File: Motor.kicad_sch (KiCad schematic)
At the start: 38 parts, among them U1 MCF8315C1VQRGFRQ1

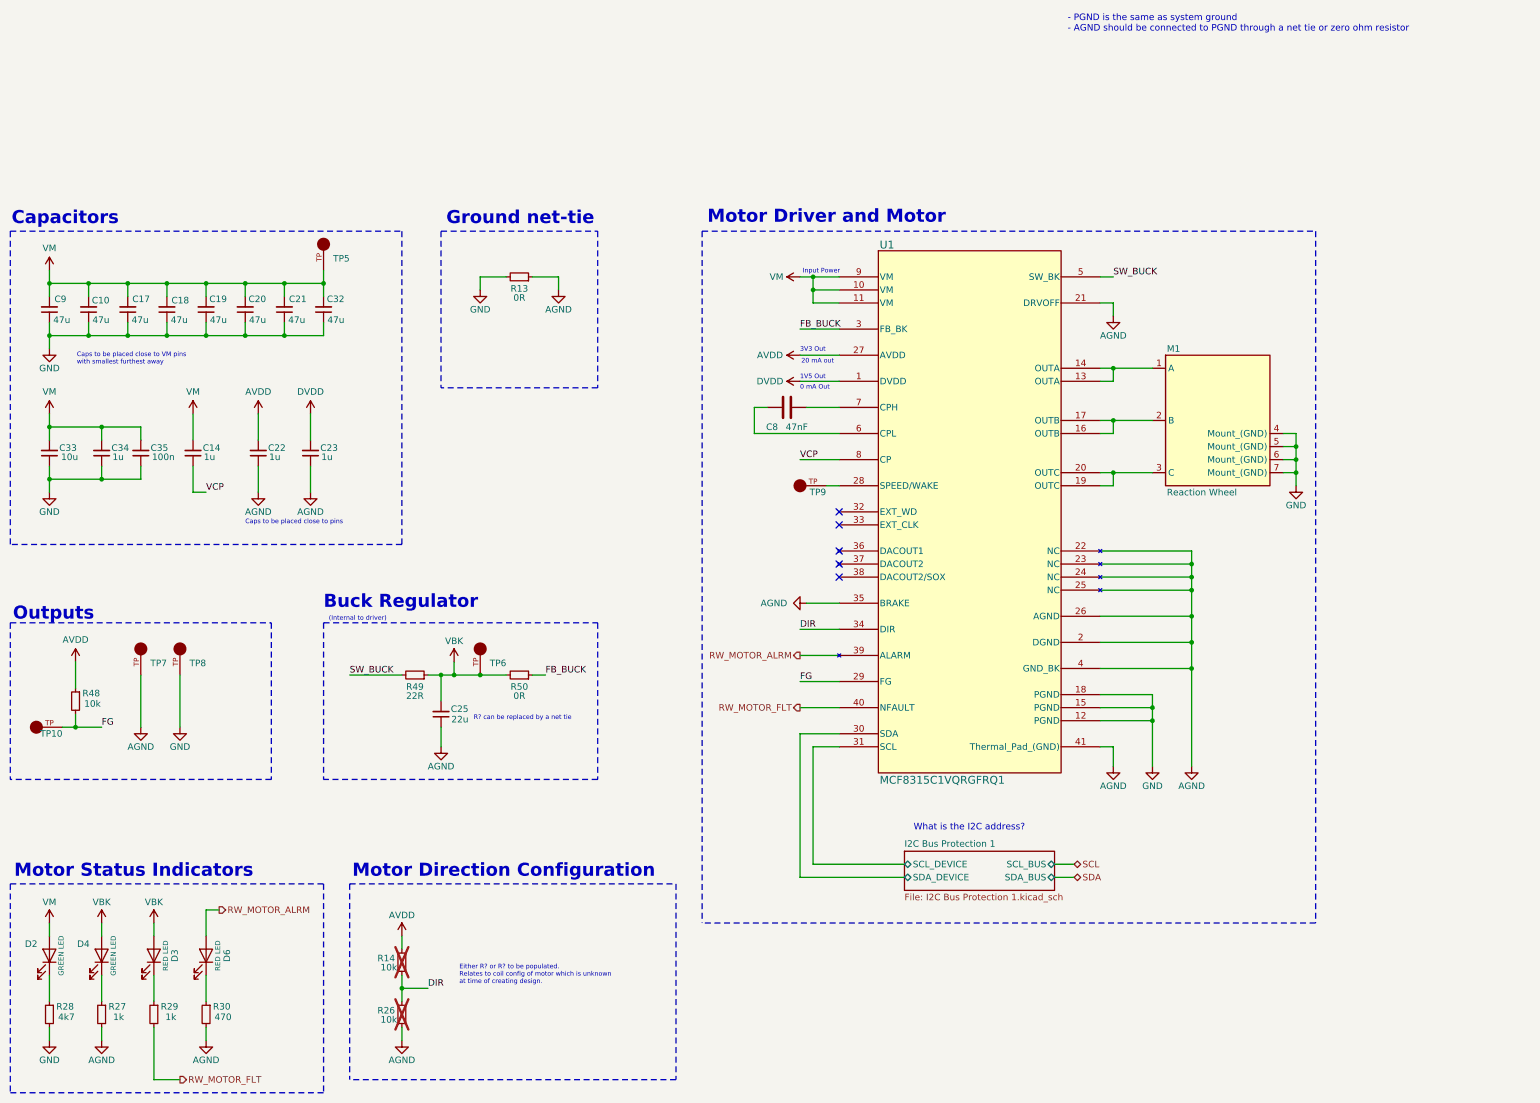
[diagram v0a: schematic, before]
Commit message: Layout mostly complete
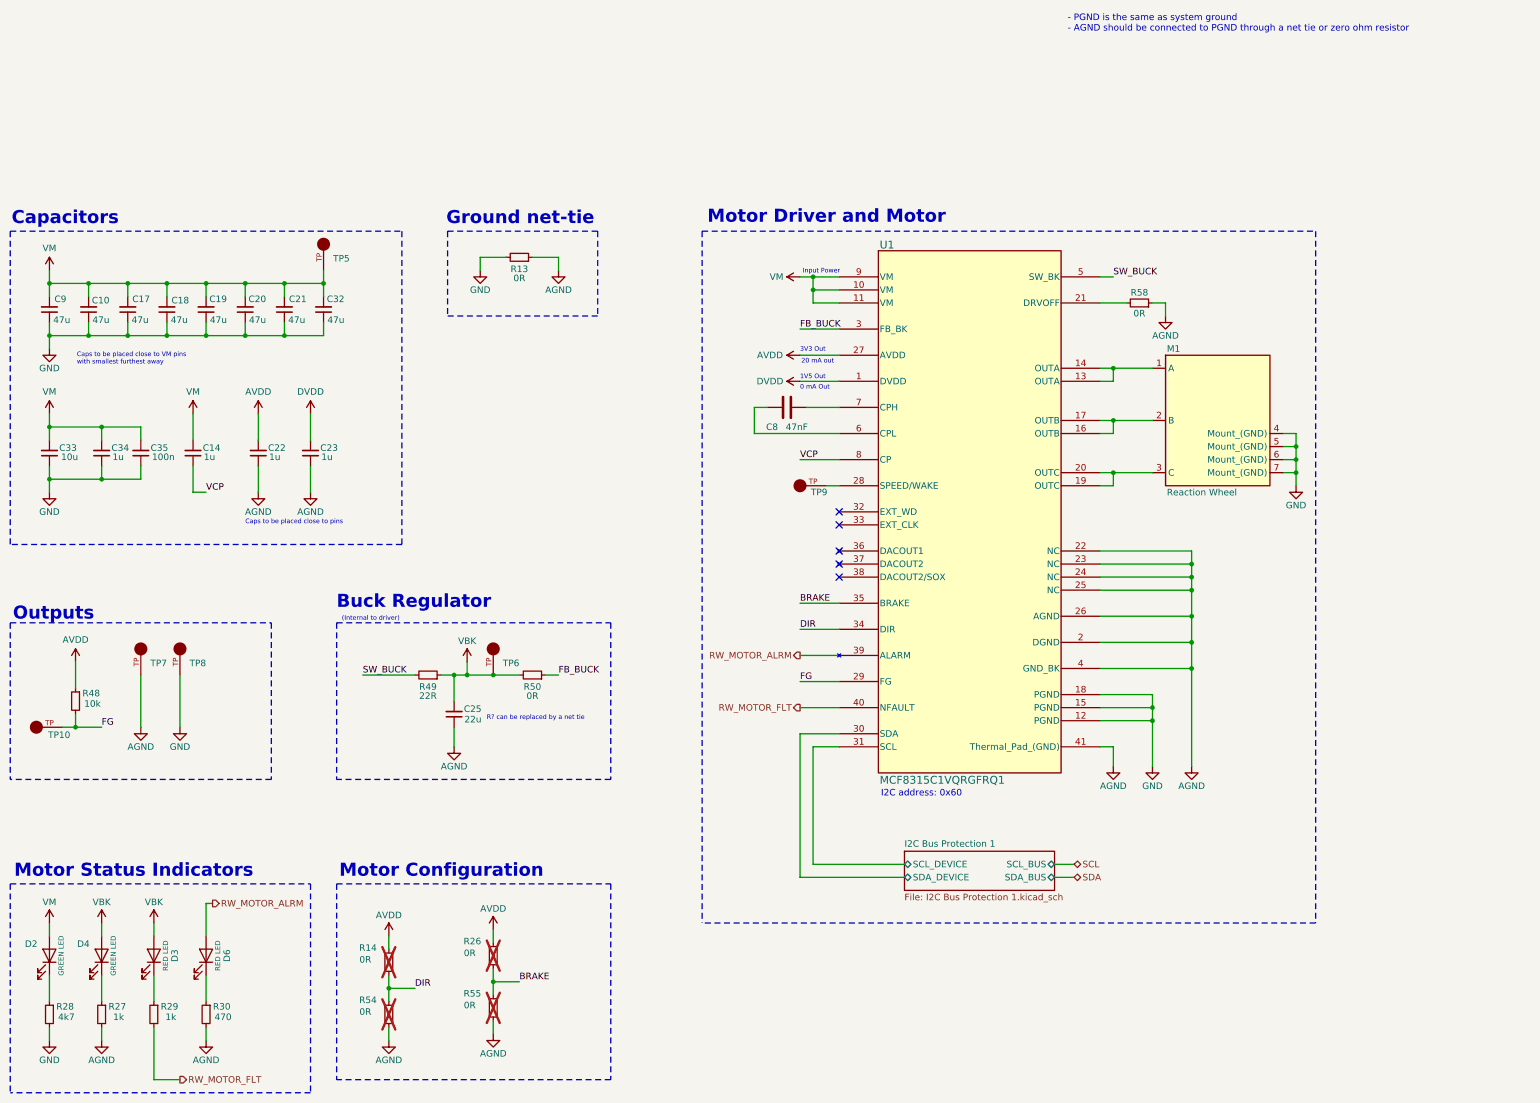
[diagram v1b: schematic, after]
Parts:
- added R54, R55, R58: 0R, Resistor_SMD:R_0402_1005Metric_Pad0.72x0.64mm_HandSolder, symbol Device:R_Small
- M1: footprint (none) -> Argus_RW_Library:Reaction_Wheel
- R14, R26: value 10k -> 0R; footprint Resistor_SMD:R_0603_1608Metric -> Resistor_SMD:R_0402_1005Metric_Pad0.72x0.64mm_HandSolder
- TP10, TP5, TP6, TP7, TP8, TP9: footprint (none) -> Argus_RW_Library:KEYSTONE_5001
- U1: footprint VQFN40_RGF_TEX -> Argus_RW_Library:VQFN40_RGF_TEX
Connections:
- net AGND: now also R54.1, R55.1, R58.1; no longer R26.1, U1.21 (DRVOFF), U1.35 (BRAKE)
- net AVDD: now also R26.2
- net DIR: now also R54.2; no longer R26.2
- new net: R58.2, U1.21 (DRVOFF)
- new net BRAKE: R26.1, R55.2, U1.35 (BRAKE)
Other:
- note added: "I2C address: 0x60"
- note added: "Motor Configuration"
- note removed: "Either R? or R? to be populated. Relates to coil config of motor which is unknown at time of creating design."
- note removed: "Motor Direction Configuration"
- note removed: "What is the I2C address?"
- title: (none) -> Argus Reaction Wheel
- moved on the sheet: C25, R13, R49, R50
